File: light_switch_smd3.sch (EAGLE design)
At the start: 17 parts, among them J2 SW1, T1 BT136, U1 LM1117

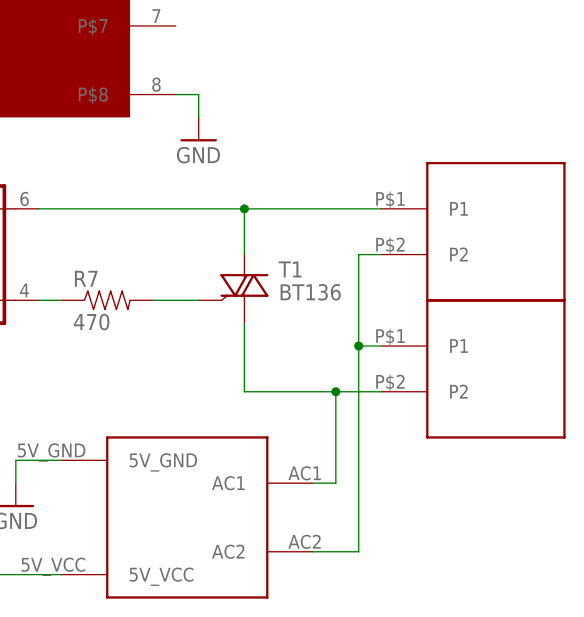
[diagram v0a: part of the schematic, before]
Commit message: light switch version 6 minor adjustments
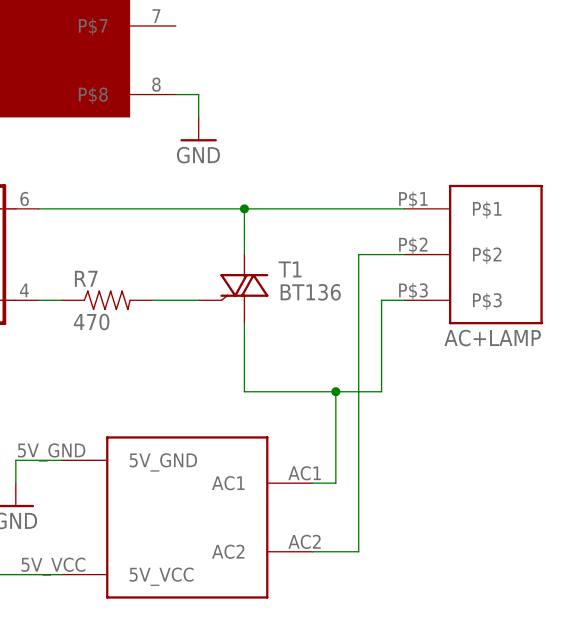
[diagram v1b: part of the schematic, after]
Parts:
- removed AC, LAMP: DG306-5.0, myblog_library:DG306-5.0
- added AC+LAMP: DG350-3.5-03P, myblog_library:DG350-3.5-03P
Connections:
- net N$11: now also AC+LAMP.P$2; no longer AC.P1, LAMP.P2
- net N$12: now also AC+LAMP.P$3; no longer AC.P2
- net N$8: now also AC+LAMP.P$1; no longer LAMP.P1
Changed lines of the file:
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@@
 <part name="U$1" library="myblog_library" deviceset="HI-LINK5V-ACDC" device=""/>
 <part name="GND4" library="supply1" deviceset="GND" device=""/>
-<part name="LAMP" library="myblog_library" deviceset="DG306-5.0" device=""/>
-<part name="AC" library="myblog_library" deviceset="DG306-5.0" device=""/>
+<part name="AC+LAMP" library="myblog_library" deviceset="DG350-3.5-03P" device=""/>
 </parts>
 <sheets>
@@
 <instance part="U$1" gate="G$1" x="78.74" y="-5.08"/>
 <instance part="GND4" gate="1" x="91.44" y="5.08"/>
-<instance part="LAMP" gate="G$1" x="144.78" y="35.56"/>
-<instance part="AC" gate="G$1" x="144.78" y="20.32"/>
+<instance part="AC+LAMP" gate="G$1" x="144.78" y="35.56" rot="MR0"/>
 </instances>
 <busses>
@@
 <pinref part="OK1" gate="-1" pin="A2"/>
 <wire x1="93.98" y1="38.1" x2="116.84" y2="38.1" width="0.1524" layer="91"/>
-<wire x1="132.08" y1="38.1" x2="116.84" y2="38.1" width="0.1524" layer="91"/>
+<pinref part="AC+LAMP" gate="G$1" pin="P$1"/>
+<wire x1="116.84" y1="38.1" x2="134.62" y2="38.1" width="0.1524" layer="91"/>
 <junction x="116.84" y="38.1"/>
-<pinref part="LAMP" gate="G$1" pin="P1"/>
 </segment>
 </net>
 <net name="N$11" class="0">
 <segment>
-<wire x1="129.54" y1="33.02" x2="129.54" y2="22.86" width="0.1524" layer="91"/>
 <pinref part="U$1" gate="G$1" pin="AC2"/>
-<wire x1="129.54" y1="22.86" x2="129.54" y2="0" width="0.1524" layer="91"/>
+<wire x1="129.54" y1="33.02" x2="129.54" y2="0" width="0.1524" layer="91"/>
 <wire x1="129.54" y1="0" x2="124.46" y2="0" width="0.1524" layer="91"/>
-<wire x1="132.08" y1="33.02" x2="129.54" y2="33.02" width="0.1524" layer="91"/>
-<wire x1="132.08" y1="22.86" x2="129.54" y2="22.86" width="0.1524" layer="91"/>
-<junction x="129.54" y="22.86"/>
-<pinref part="LAMP" gate="G$1" pin="P2"/>
-<pinref part="AC" gate="G$1" pin="P1"/>
+<pinref part="AC+LAMP" gate="G$1" pin="P$2"/>
+<wire x1="134.62" y1="33.02" x2="129.54" y2="33.02" width="0.1524" layer="91"/>
 </segment>
 </net>
@@
 <pinref part="U$1" gate="G$1" pin="AC1"/>
 <wire x1="127" y1="7.62" x2="124.46" y2="7.62" width="0.1524" layer="91"/>
+<pinref part="AC+LAMP" gate="G$1" pin="P$3"/>
+<wire x1="134.62" y1="27.94" x2="132.08" y2="27.94" width="0.1524" layer="91"/>
+<wire x1="132.08" y1="27.94" x2="132.08" y2="17.78" width="0.1524" layer="91"/>
 <wire x1="132.08" y1="17.78" x2="127" y2="17.78" width="0.1524" layer="91"/>
 <junction x="127" y="17.78"/>
-<pinref part="AC" gate="G$1" pin="P2"/>
 </segment>
 </net>
